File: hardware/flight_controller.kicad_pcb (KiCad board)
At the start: 6 copper layers, 50 x 50 mm, 81 parts, among them IC2 STM32F722RET6, IC3 W25Q128JVSIQ, J1 Conn_01x03, J2 Conn_01x08, J3 Conn_01x04, J4 Conn_01x04, J5 Conn_01x04, J6 USB4105-GF-A-060, Q1 TPRT9013-33GB, SW2 SW_SPST, U1 BMP581, U2 MP9943GQ-Z, U3 USBLC6-2P6, U4 MP9943GQ-Z, Y2 X322525MOB4SI

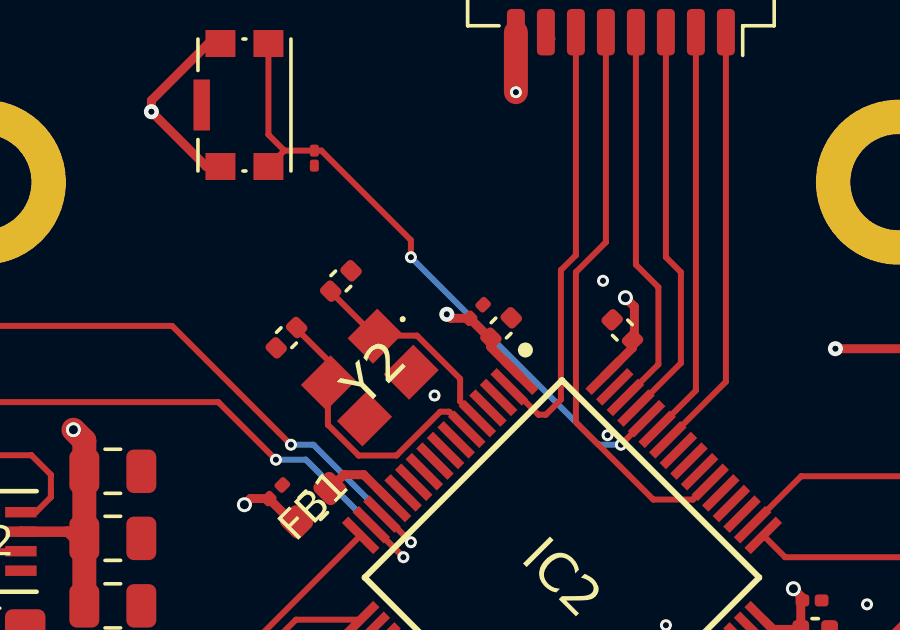
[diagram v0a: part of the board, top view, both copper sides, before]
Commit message: fix errors
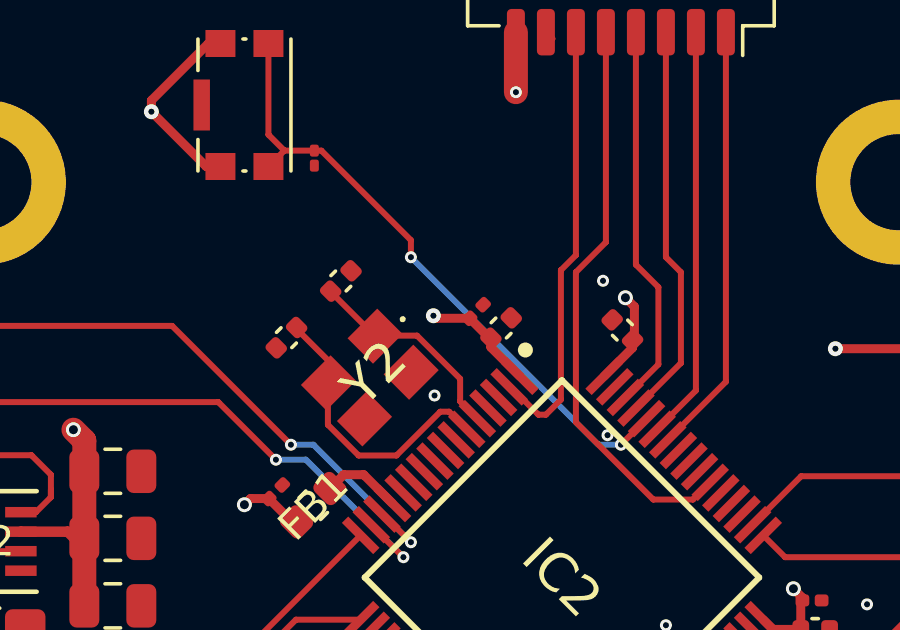
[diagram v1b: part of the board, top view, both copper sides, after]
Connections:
- IC2 pad 44: /USB_DN -> /USB_D_DN
- IC2 pad 45: /USB_DP -> /USB_D_DP
- R10 pad 2: /USB_DP -> /USB_D_DP
- R9 pad 2: /USB_DN -> /USB_D_DN
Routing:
- net /USB_D_DN: track 0.00 -> 9.58 mm
- net /USB_DN: track 13.3 -> 3.74 mm
- net /USB_D_DP: track 0.00 -> 8.75 mm
- net /USB_DP: track 12.1 -> 3.30 mm
